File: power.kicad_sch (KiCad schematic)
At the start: 24 parts, among them U7 AP63203WU, U9 TPS62130

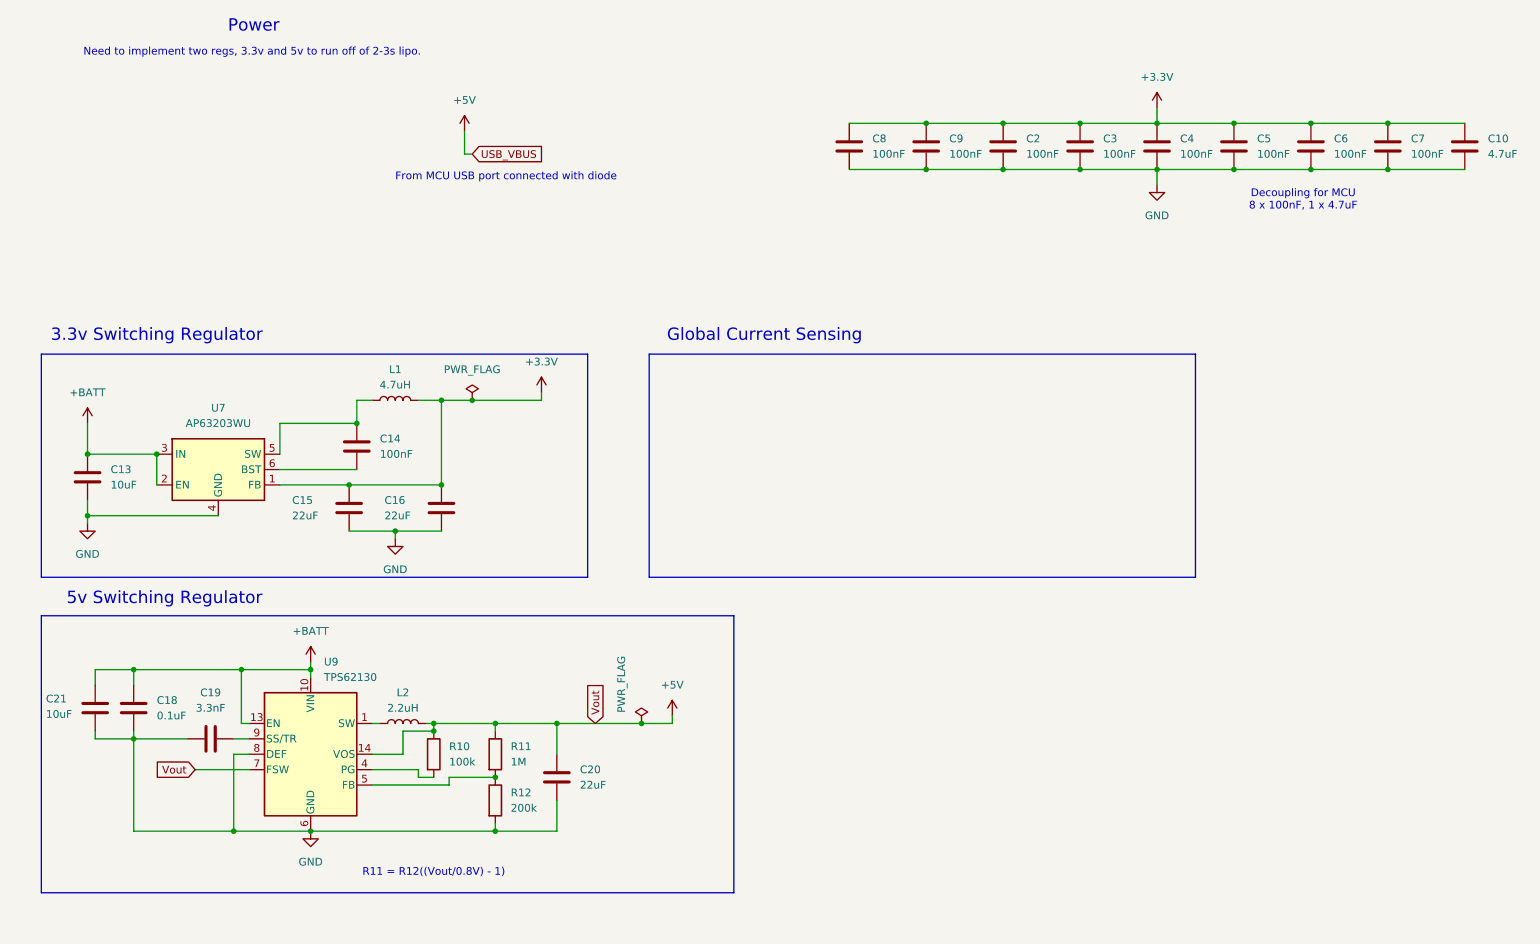
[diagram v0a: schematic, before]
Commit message: branches
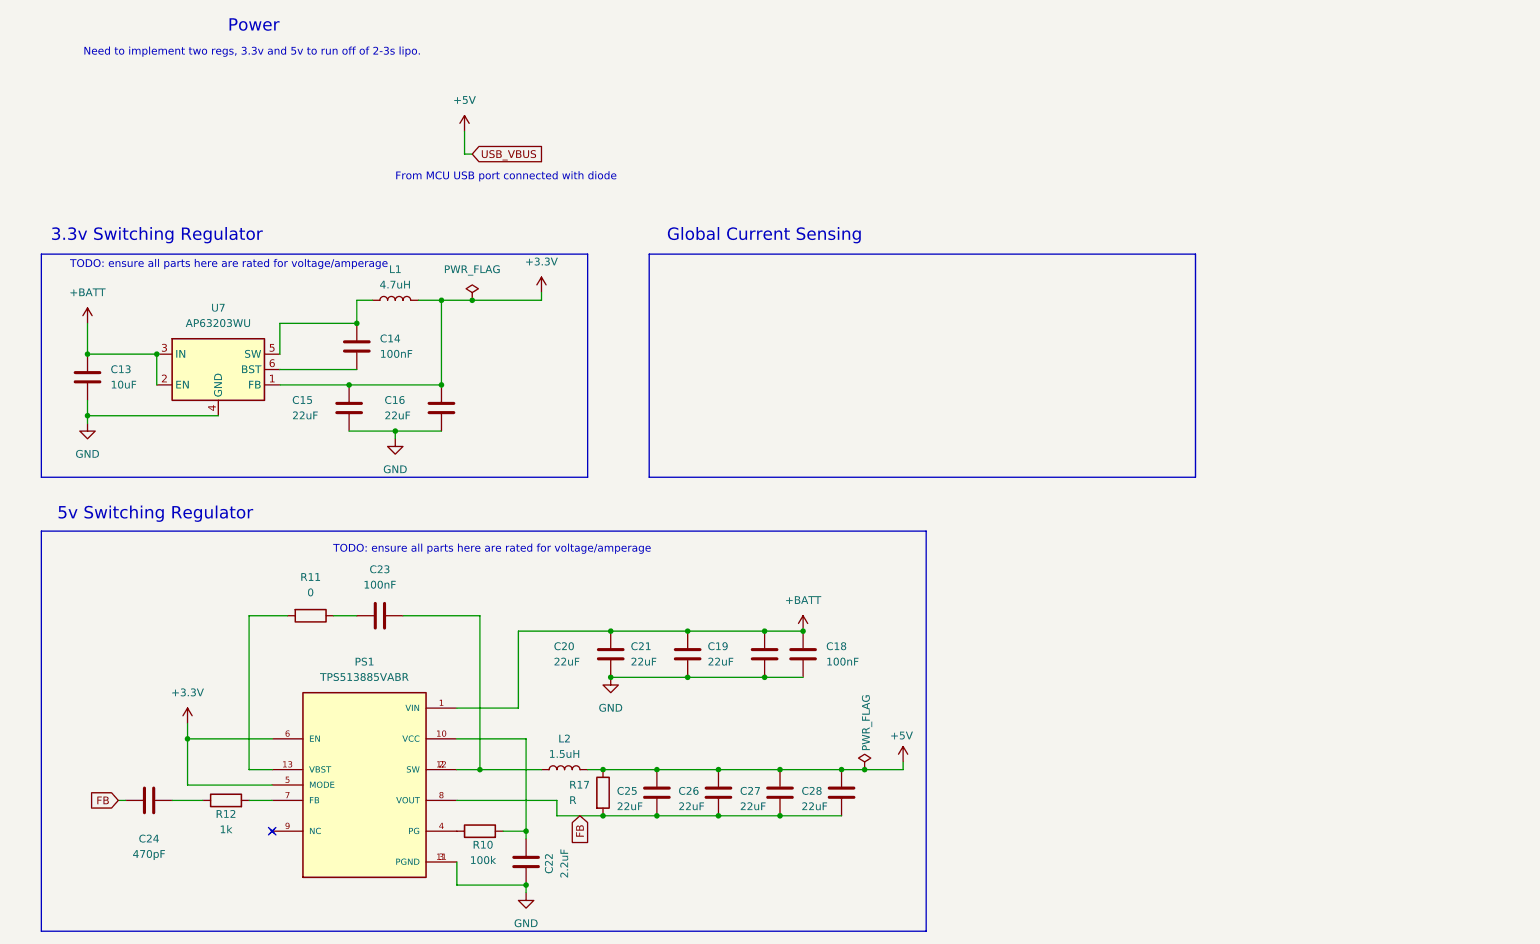
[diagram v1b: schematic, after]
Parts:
- removed C10: 4.7uF, Capacitor_SMD:C_0603_1608Metric, symbol Device:C
- removed C2, C3, C4, C5, C6, C7, C8, C9: 100nF, Capacitor_SMD:C_0402_1005Metric, symbol Device:C
- removed U9: TPS62130, Package_DFN_QFN:VQFN-16-1EP_3x3mm_P0.5mm_EP1.68x1.68mm_ThermalVias, symbol Regulator_Switching:TPS62130
- added C22: 2.2uF, Capacitor_SMD:C_0603_1608Metric, symbol Device:C
- added C23: 100nF, Capacitor_SMD:C_0402_1005Metric, symbol Device:C
- added C24: 470pF, Capacitor_SMD:C_0402_1005Metric, symbol Device:C
- added C25, C26, C27, C28: 22uF, Capacitor_SMD:C_1206_3216Metric, symbol Device:C
- added PS1: TPS513885VABR, TPS513885VABR:CONV_TPS513885VABR, symbol TPS513885VABR:TPS513885VABR
- added R17: R, symbol Device:R
- C18: value 0.1uF -> 100nF
- C19: value 3.3nF -> 22uF; footprint Capacitor_SMD:C_0402_1005Metric -> Capacitor_SMD:C_1206_3216Metric
- C21: value 10uF -> 22uF; footprint Capacitor_SMD:C_0805_2012Metric -> Capacitor_SMD:C_1206_3216Metric
- L2: value 2.2uH -> 1.5uH
- R11: value 1M -> 0; footprint Resistor_SMD:R_0603_1608Metric -> (none)
- R12: value 200k -> 1k; footprint Resistor_SMD:R_0603_1608Metric -> Resistor_SMD:R_0402_1005Metric
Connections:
- net +3.3V: now also PS1.5 (MODE), PS1.6 (EN)
- net +5V: now also C25.1, C26.1, C27.1, C28.1, R17.1; no longer C20.1, R10.1, R11.1
- net +BATT: now also C18.1, C19.1, C20.1, C21.1, PS1.1 (VIN); no longer C18.2, C21.2
- net GND: now also C18.2, C21.2, C22.1, PS1.11 (PGND), PS1.3 (PGND); no longer C18.1, C21.1, R12.2
- net at R11.2: now also PS1.13 (VBST); no longer R12.1
- net at L2.1: now also C23.2, PS1.12 (SW), PS1.2 (SW)
- net at R10.2: now also C22.2, PS1.10 (VCC)
- new net: PS1.4 (PG), R10.1
- new net: PS1.7 (FB), R12.2
- new net: C24.2, R12.1
- new net: C23.1, R11.1
- new net FB: C24.1, C25.2, C26.2, C27.2, C28.2, PS1.8 (VOUT), R17.2
- no-connect marks 0 -> 1
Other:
- note added: "TODO: ensure all parts here are rated for voltage/amperage"
- note removed: "Decoupling for MCU 8 x 100nF, 1 x 4.7uF"
- note removed: "R11 = R12((Vout/0.8V) - 1)"
- moved on the sheet: C13, C14, C15, C16, L1, U7
